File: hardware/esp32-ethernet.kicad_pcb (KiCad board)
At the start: 4 copper layers, 80 x 40 mm, 126 parts, among them J101 USB-C-2, P101 EXT_HEADER, P201 CON-SENSOR2, P202 CON-SENSOR2, P203 CON-SENSOR2, P204 CON-SENSOR2, P205 CON-SENSOR2, P206 CON-SENSOR2, P301 POE, P302 RJPSL-001TA1, Q101 BC817, Q102 BC817, SW101 B3U-1000P, SW102 B3U-1000P, U101 82400152, U102 AZ1117E-3.3V, U103 CP2102N-A02-GQFN24R, U104 ESP32-WROVER-E, U201 74AHC244, U202 74AHC244, U203 74AHC244, U204 SN74LV138AD, U301 KSZ80X1RNA, X301 25Mhz

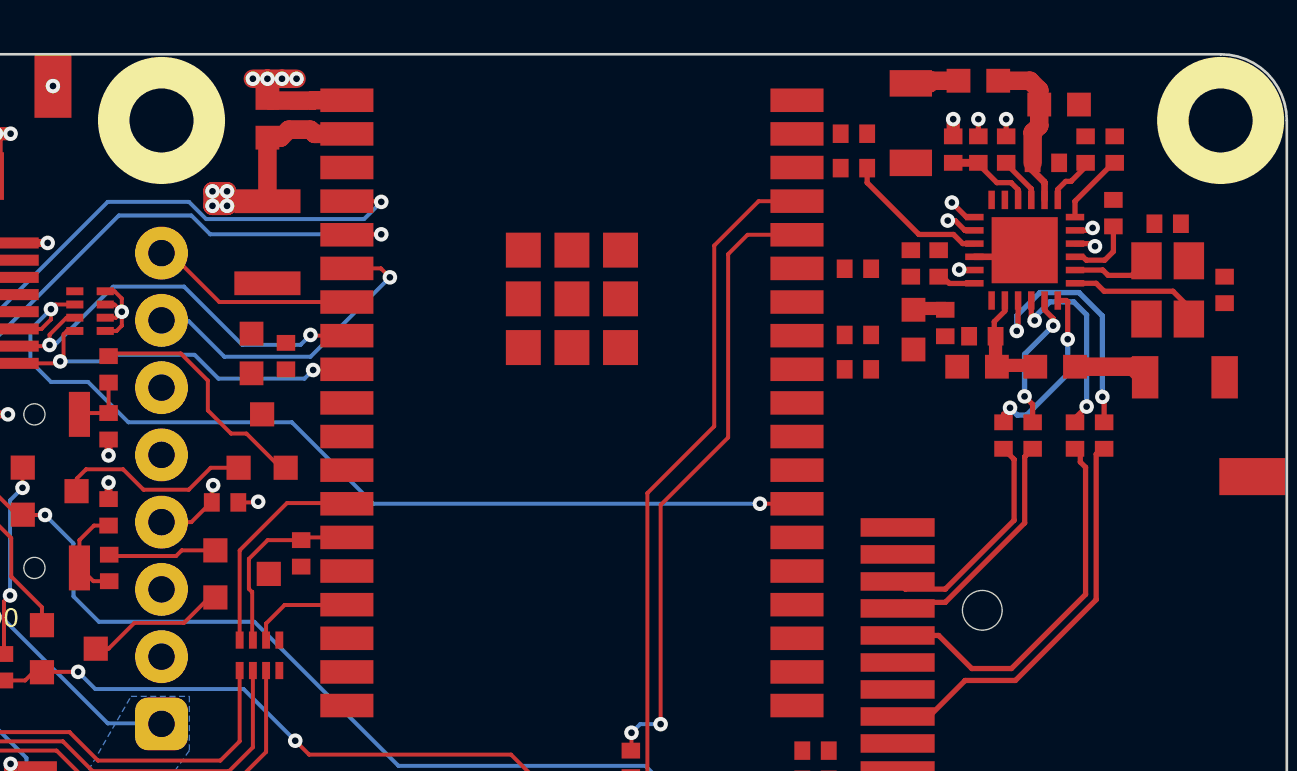
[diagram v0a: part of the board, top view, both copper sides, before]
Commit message: more routing
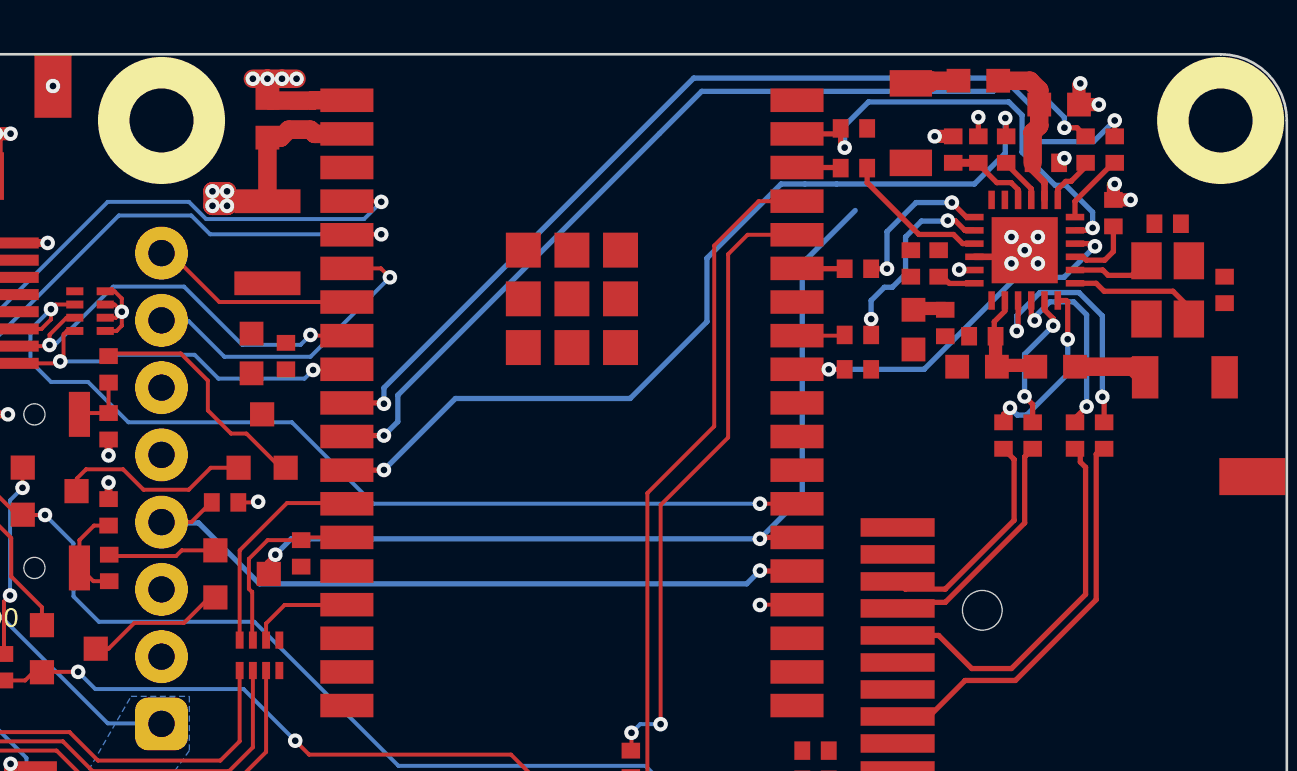
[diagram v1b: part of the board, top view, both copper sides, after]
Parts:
- moved R310 0.20 mm to (177.4, 126.5)
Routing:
- net RMII_RXD1: track 0.00 -> 37.5 mm, vias 0 -> 2
- net ESP_IO0: track 0.65 -> 35.4 mm, vias 1 -> 3
- net RMII_RXD0: track 0.00 -> 34.6 mm, vias 0 -> 2
- net RMII_CRS: track 0.65 -> 33.3 mm, vias 1 -> 2
- net LED_GREEN: track 2.88 -> 27.4 mm
- net RMII_MDC: track 0.70 -> 16.9 mm, vias 1 -> 2
- net RMII_MDIO: track 0.80 -> 14.6 mm, vias 1 -> 2
- net Net-(R304-Pad1): track 1.16 -> 7.42 mm, vias 1 -> 2
- net GND: track 114.7 -> 120.6 mm, vias 119 -> 129
- net Net-(R306-Pad1): track 1.08 -> 6.58 mm, vias 1 -> 2
- net RMII_TX_EN: track 0.00 -> 3.11 mm
- net RMII_TXD0: track 0.00 -> 1.81 mm
- net RMII_TXD1: track 0.00 -> 1.61 mm
- net LED_BLUE: track 0.00 -> 1.41 mm, vias 0 -> 1
